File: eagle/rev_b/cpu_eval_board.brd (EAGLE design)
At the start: 114.3 x 88.9 mm, 112 parts, among them IC1 6N138S-TA1, IC2 6N138S-TA1, IC5 74HC595D, Q1 BC337, SW1 Encoder, SW2 Encoder, U1 24LC512, Y1 8MHz

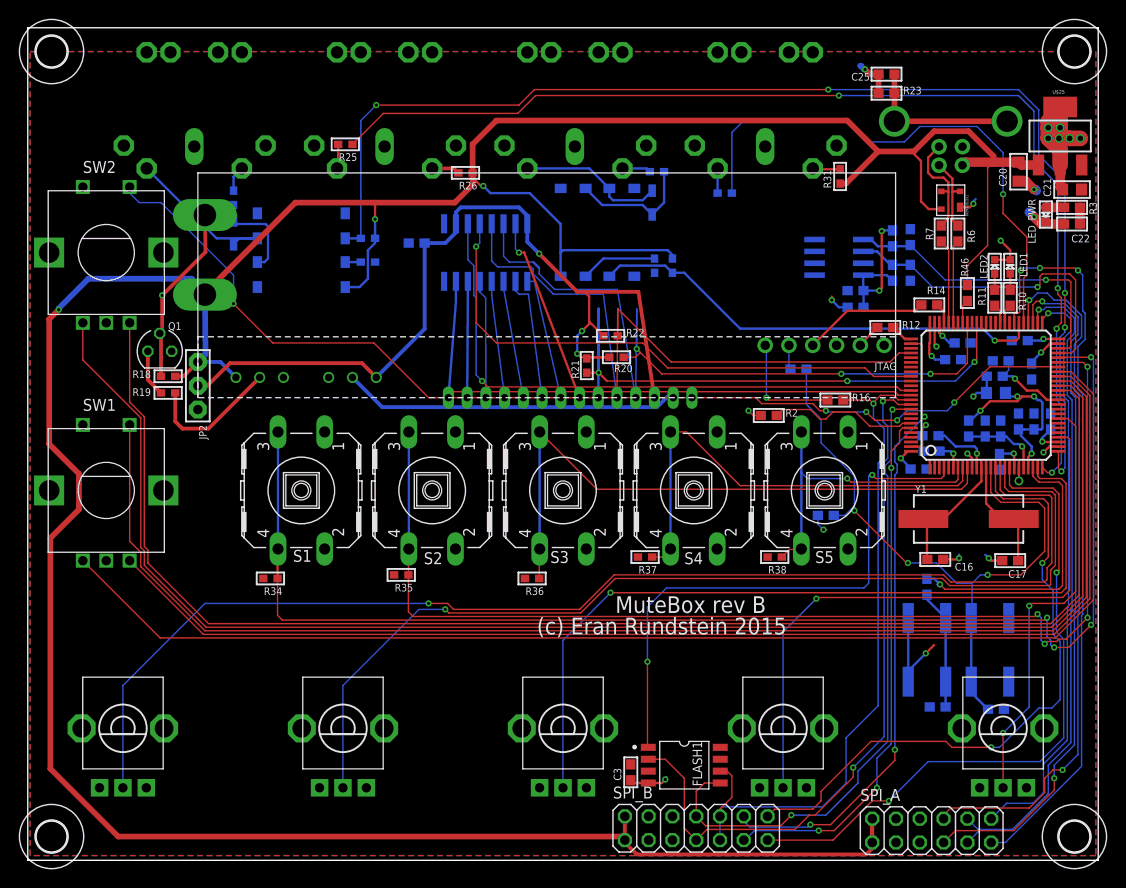
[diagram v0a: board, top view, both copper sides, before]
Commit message: cpu_eval_board rev b sent to oshpark
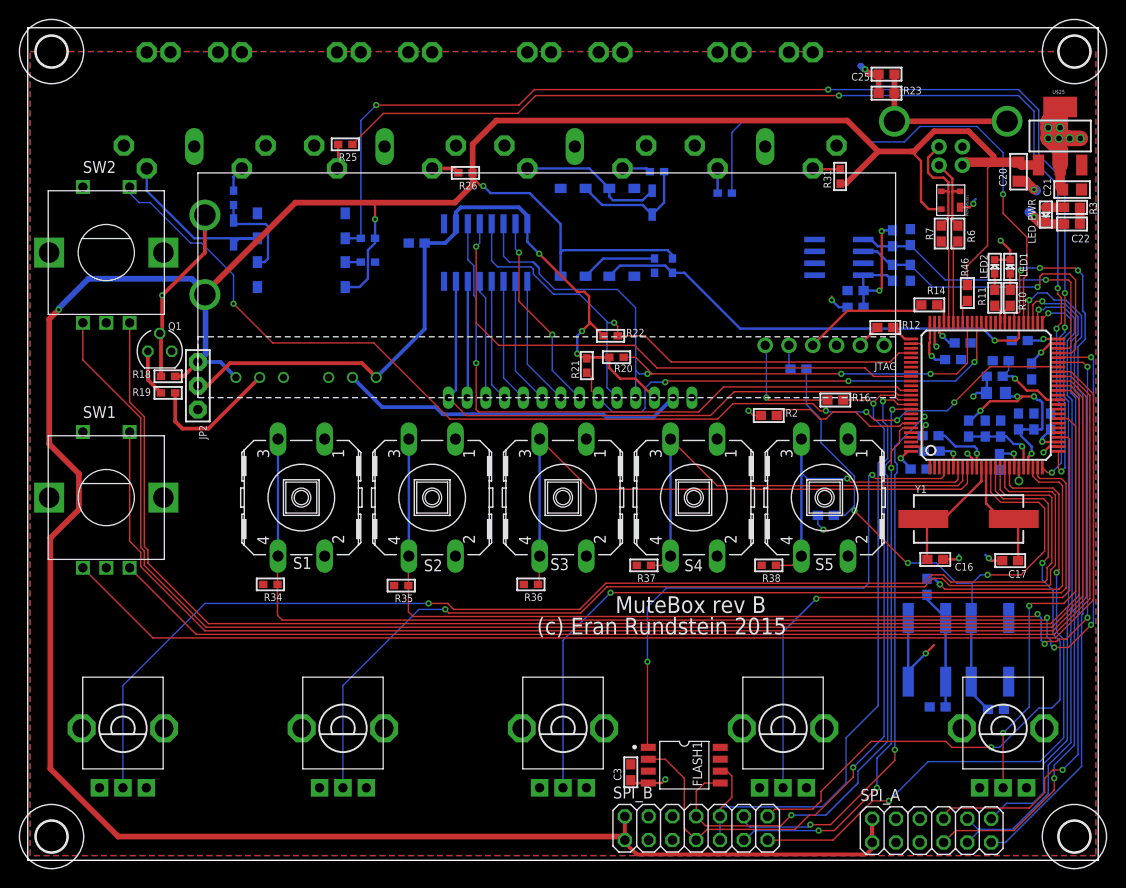
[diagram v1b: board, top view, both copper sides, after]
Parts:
- moved R35 1.14 mm to (39.9, 29.3)
- moved R38 1.09 mm to (79.1, 31.5)
- moved R37 0.90 mm to (65.8, 31.5)
- moved S1 0.76 mm to (29.2, 38.7)
- moved S2 0.76 mm to (43.2, 38.7)
- moved S3 0.76 mm to (57.1, 38.7)
- moved S4 0.76 mm to (71.1, 38.7)
- moved S5 0.76 mm to (85.1, 38.7)
- moved SW1 0.76 mm to (8.38, 38.7)
- moved R36 0.65 mm to (53.7, 29.5)
- moved R34 0.64 mm to (25.9, 29.5)
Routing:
- net LCD_RW: track 75.3 -> 63.1 mm, vias 0 -> 1
- net LCD_RS: track 86.1 -> 74.0 mm
- net LCD_E1: track 63.2 -> 51.7 mm
- net LCD_VD: track 96.0 -> 85.3 mm
- net LCD_SER_SCLK: track 63.6 -> 68.0 mm
- net N$27: track 17.7 -> 19.1 mm
- net SCS_D5: track 114.1 -> 115.5 mm
- net LCD_D0: track 20.4 -> 21.4 mm, vias 1 -> 2
- net LCD_D7: track 63.1 -> 64.1 mm
- net SCS_D2: track 146.0 -> 145.3 mm
- net SCS_D6: track 126.0 -> 125.3 mm
- net SCS_D7: track 142.9 -> 142.1 mm
- net SCS_D8: track 33.5 -> 34.2 mm
- net LCD_D3: track 12.6 -> 13.3 mm
